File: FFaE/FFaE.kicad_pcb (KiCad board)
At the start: 2 copper layers, 60 x 85 mm, 69 parts, among them J1 Conn_01x02_Pin, Q1 BC337, U1 LM741, U2 PT2399, U3 L7805, U4 L7809, U5 LM741, U6 LM741

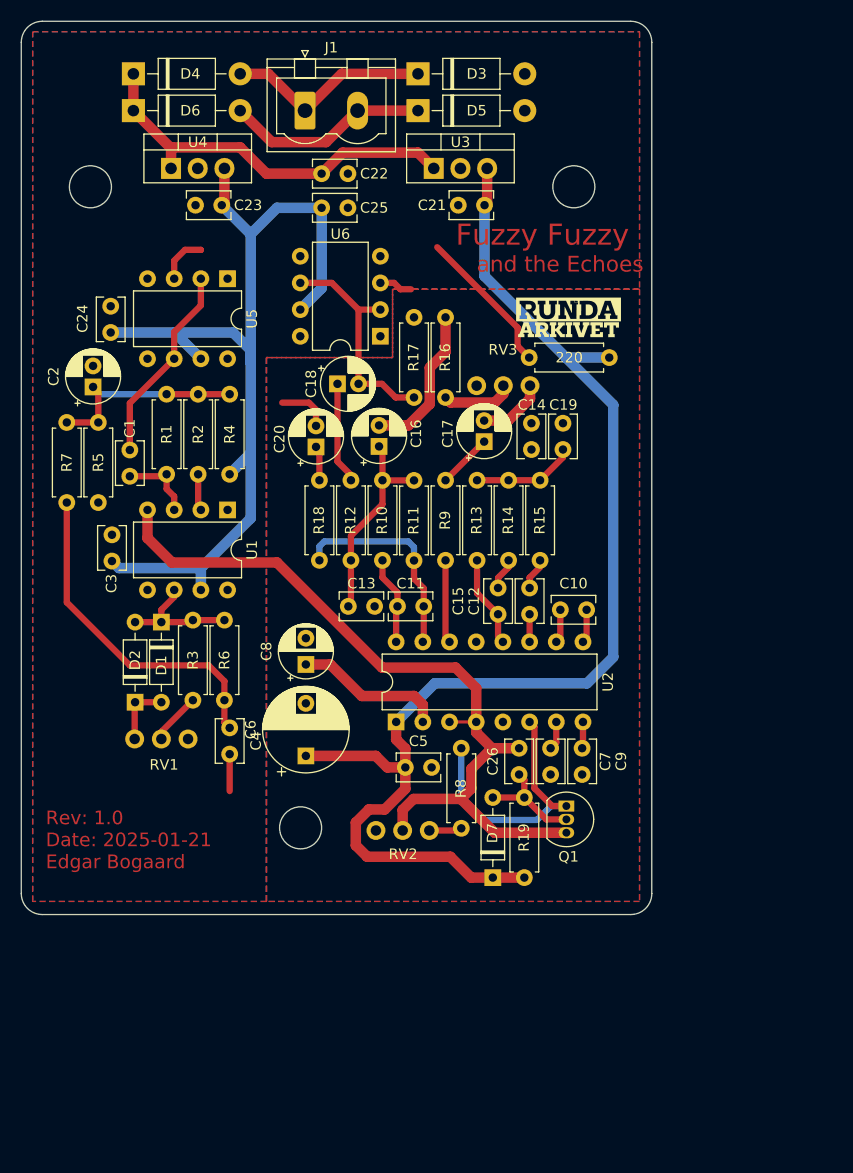
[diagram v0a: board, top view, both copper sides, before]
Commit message: PCB v0
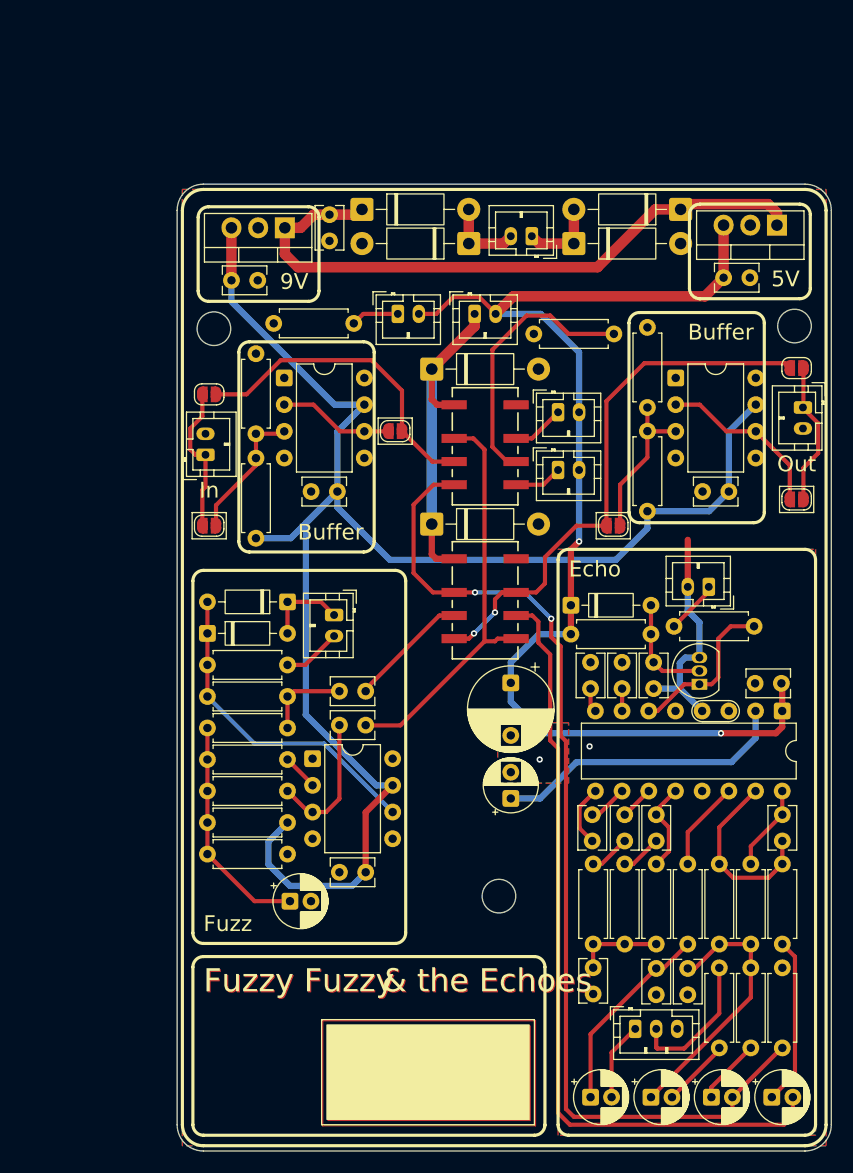
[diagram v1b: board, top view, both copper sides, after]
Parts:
- removed 220: 3.3k, Resistor_THT:R_Axial_DIN0207_L6.3mm_D2.5mm_P7.62mm_Horizontal
- removed G*** (x2): LOGO, LOGO
- removed the REF** at (82.2, 40.2)
- removed the REF** at (36.2, 40.2)
- removed the REF** at (56.2, 101.2)
- added ?: , , F.Cu at (48.0, 53.8)
- added ?: , , F.Cu at (103.2, 53.5)
- added D10: LED, Connector_JST:JST_PH_B2B-PH-K_1x02_P2.00mm_Vertical, F.Cu at (65.5, 52.3)
- added D11: LED, Connector_JST:JST_PH_B2B-PH-K_1x02_P2.00mm_Vertical, F.Cu at (80.8, 61.7)
- added D12: LED, Connector_JST:JST_PH_B2B-PH-K_1x02_P2.00mm_Vertical, F.Cu at (80.8, 67.2)
- added D8: 1N4007, Diode_THT:D_DO-41_SOD81_P10.16mm_Horizontal, F.Cu at (68.7, 57.6)
- added D9: 1N4007, Diode_THT:D_DO-41_SOD81_P10.16mm_Horizontal, F.Cu at (68.7, 72.3)
- added J10: Input_Jack, Connector_JST:JST_PH_B2B-PH-K_1x02_P2.00mm_Vertical, F.Cu at (47.2, 65.8)
- added J11: Output_Jack, Connector_JST:JST_PH_B2B-PH-K_1x02_P2.00mm_Vertical, F.Cu at (104.0, 61.2)
- added JP1: SolderJumper_2_Open, Jumper:SolderJumper-2_P1.3mm_Open_RoundedPad1.0x1.5mm, F.Cu at (47.5, 72.5)
- added JP2: SolderJumper_2_Open, Jumper:SolderJumper-2_P1.3mm_Open_RoundedPad1.0x1.5mm, F.Cu at (47.5, 60.0)
- added JP3: SolderJumper_2_Open, Jumper:SolderJumper-2_P1.3mm_Open_RoundedPad1.0x1.5mm, F.Cu at (103.5, 70.0)
- added JP4: SolderJumper_2_Open, Jumper:SolderJumper-2_P1.3mm_Open_RoundedPad1.0x1.5mm, F.Cu at (103.5, 57.5)
- added JP5: SolderJumper_2_Open, Jumper:SolderJumper-2_P1.3mm_Open_RoundedPad1.0x1.5mm, F.Cu at (65.2, 63.5)
- added JP6: SolderJumper_2_Open, Jumper:SolderJumper-2_P1.3mm_Open_RoundedPad1.0x1.5mm, F.Cu at (86.0, 72.5)
- added R20: 100k, Resistor_THT:R_Axial_DIN0207_L6.3mm_D2.5mm_P7.62mm_Horizontal, F.Cu at (52.0, 73.7)
- added R21: 100k, Resistor_THT:R_Axial_DIN0207_L6.3mm_D2.5mm_P7.62mm_Horizontal, F.Cu at (89.2, 71.1)
- added R22: 100k, Resistor_THT:R_Axial_DIN0207_L6.3mm_D2.5mm_P7.62mm_Horizontal, F.Cu at (52.0, 63.8)
- added R23: 100k, Resistor_THT:R_Axial_DIN0207_L6.3mm_D2.5mm_P7.62mm_Horizontal, F.Cu at (89.2, 61.2)
- added R24: 220R, Resistor_THT:R_Axial_DIN0207_L6.3mm_D2.5mm_P7.62mm_Horizontal, F.Cu at (86.1, 54.2)
- added R25: 220R, Resistor_THT:R_Axial_DIN0207_L6.3mm_D2.5mm_P7.62mm_Horizontal, F.Cu at (53.7, 53.2)
- added REF**: MountingHole_3.2mm_M3, MountingHole:MountingHole_3.2mm_M3, F.Cu at (75.1, 107.8)
- added SW1: Shoegaze, Connector_JST:JST_PH_B2B-PH-K_1x02_P2.00mm_Vertical, F.Cu at (72.8, 52.3)
- added U7: UB2-5NUN, KiCAD_lib:UB2-5NUN, F.Cu at (73.8, 64.9)
- added U8: UB2-5NUN, KiCAD_lib:UB2-5NUN, F.Cu at (73.8, 79.6)
- J1: value Conn_01x02_Pin -> DC_in; footprint Connector_Phoenix_MSTB:PhoenixContact_MSTBVA_2,5_2-G_1x02_P5.00mm_Vertical -> Connector_JST:JST_PH_B2B-PH-K_1x02_P2.00mm_Vertical
- RV1, RV2: footprint Potentiometer_THT:Potentiometer_Vishay_148-149_Single_Horizontal -> Connector_JST:JST_PH_B2B-PH-K_1x02_P2.00mm_Vertical
- RV3: footprint Potentiometer_THT:Potentiometer_Vishay_148-149_Single_Horizontal -> Connector_JST:JST_PH_B3B-PH-K_1x03_P2.00mm_Vertical
- moved C18 76.6 mm to (95.3, 126.9)
- moved C20 75.6 mm to (101.1, 126.9), turned to 0 degrees
- moved R17 71.1 mm to (102.1, 114.6)
- moved C16 67.1 mm to (89.6, 126.9), turned to 0 degrees
- moved C17 63.2 mm to (83.8, 126.9), turned to 0 degrees
- moved RV3 62.0 mm to (88.1, 120.4), turned to 0 degrees
- moved R16 60.2 mm to (96.1, 114.6), turned to -90 degrees
- moved C14 55.7 mm to (90.1, 117.1), turned to 90 degrees
- moved R12 54.3 mm to (99.1, 114.6), turned to -90 degrees
- moved D4 53.6 mm to (92.4, 42.4), turned to 180 degrees
- moved R18 52.7 mm to (102.1, 104.7), turned to -90 degrees
- moved C2 52.4 mm to (55.2, 108.2), turned to 0 degrees
- moved C19 49.4 mm to (84.1, 114.6), turned to -90 degrees
- moved C13 47.5 mm to (93.1, 117.1), turned to 90 degrees
- moved R10 45.4 mm to (99.1, 104.7), turned to -90 degrees
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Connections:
- C1 pad 1: /Fuzz/Input -> /Fuzz_input
- C18 pad 2: /Echo/Input -> /Echo_input
- C20 pad 2: /Echo/Output -> /Echo_output
- C4 pad 1: /Fuzz/Output -> /Fuzz_output
- R17 pad 2: /Echo/Input -> /Echo_input
- RV1 pad 1: unconnected-(RV1-Pad1) -> Net-(D1-A)
- RV2 pad 1: unconnected-(RV2-Pad1) -> Net-(R8-Pad1)
- U5 pad 2: /Fuzz/Input -> /Input Buffer/Output
- U5 pad 3: /Input buffer 1/Input -> /Input Buffer/Input
- U5 pad 6: /Fuzz/Input -> /Input Buffer/Output
- U6 pad 2: /Echo/Input -> /Output Buffer/Output
- U6 pad 3: /Input buffer 2/Input -> /Output Buffer/Input
- U6 pad 6: /Echo/Input -> /Output Buffer/Output
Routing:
- net /Echo_input: track 0.00 -> 97.6 mm, vias 0 -> 2
- net /Echo_output: track 0.00 -> 74.8 mm
- net +9V: track 92.0 -> 154.7 mm
- net GND: track 76.7 -> 21.7 mm
- net /Output: track 0.00 -> 52.1 mm, vias 0 -> 2
- net /Fuzz_input: track 0.00 -> 39.3 mm
- net Net-(D8-K): track 0.00 -> 32.1 mm
- net /Input: track 0.00 -> 30.3 mm
- net Net-(R24-Pad1): track 0.00 -> 25.7 mm
- net Net-(C4-Pad2): track 32.3 -> 8.15 mm
- net Net-(D4-K): track 38.0 -> 61.9 mm
- net /Echo/Input: track 21.6 -> 0.00 mm
- net /Fuzz/Input: track 19.1 -> 0.00 mm
- net Net-(D1-K): track 12.1 -> 31.2 mm
- net /Output Buffer/Output: track 0.00 -> 16.5 mm
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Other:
- board size 60 x 85 mm -> 62.2 x 92 mm
- board text added: "& the Echoes"
- board text added: "5V"
- board text added: "9V"
- board text added: "Buffer"
- board text added: "Echo"
- board text added: "Fuzz"
- board text added: "In"
- board text added: "Out"
- board text added: "R1"
- board text removed: "Rev: 1.0 Date: 2025-01-21 Edgar Bogaard"
- board text removed: "and the Echoes"
